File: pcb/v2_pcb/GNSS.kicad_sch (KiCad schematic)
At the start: 22 parts, among them J900 U.FL / Beitian BT-T076, U900 UM980

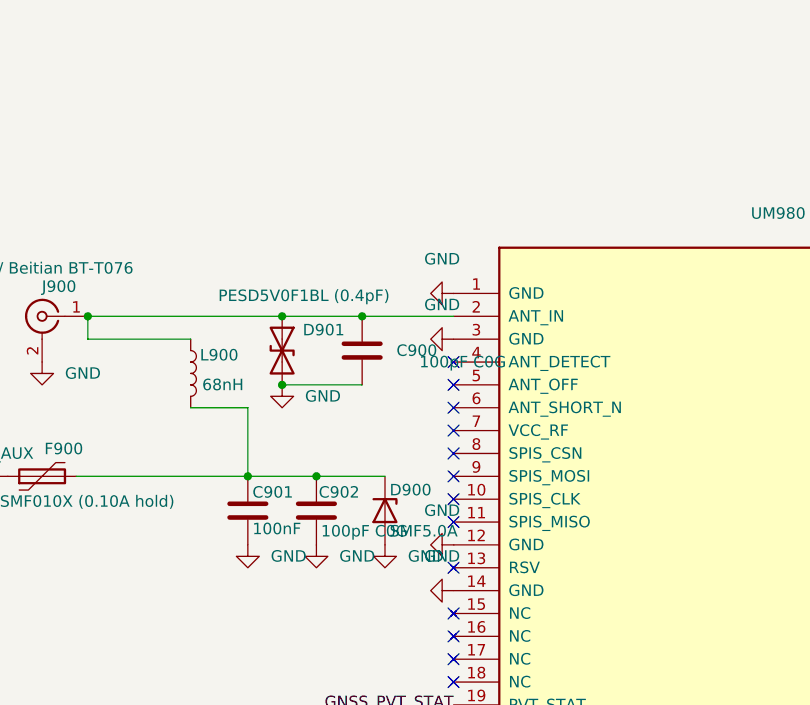
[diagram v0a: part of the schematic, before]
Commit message: fix minor
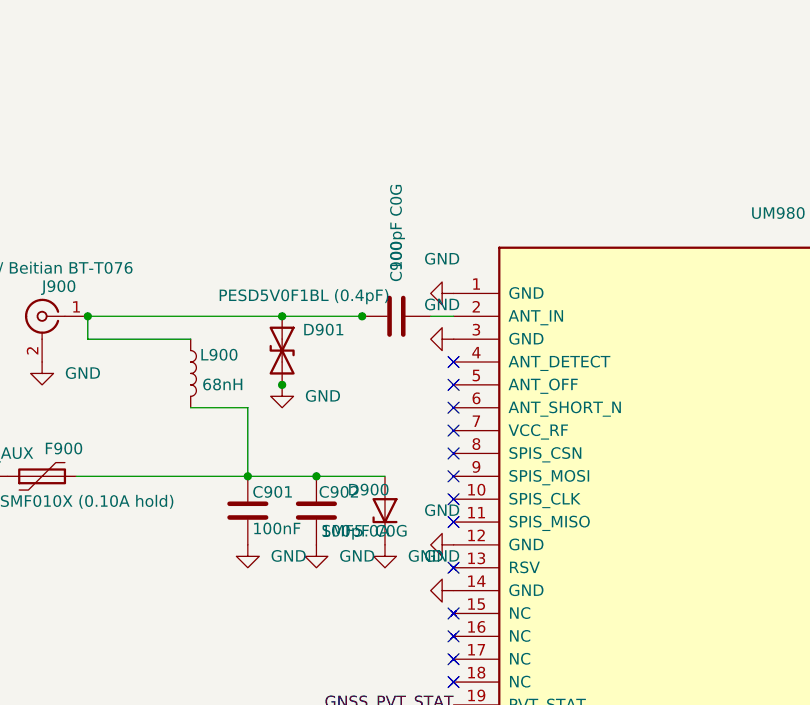
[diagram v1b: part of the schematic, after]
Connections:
- net GND: now also D900.1 (K); no longer C900.2, D900.2 (A)
- net at C901.1, C902.1, F900.2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: now also D900.2 (A); no longer D900.1 (K)
- net at C900.1, D901.1 (A1), J900.1 (In)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: no longer U900.2 (ANT_IN)
- new net: C900.2, U900.2 (ANT_IN)
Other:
- moved on the sheet: C900, D900
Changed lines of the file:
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@@
 	(wire
 		(pts
-			(xy 162.56 104.14) (xy 171.45 104.14)
-		)
-		(stroke
-			(width 0)
-			(type default)
-		)
-	)
-	(wire
-		(pts
 			(xy 323.85 146.05) (xy 349.25 146.05)
 		)
@@
 	(wire
 		(pts
-			(xy 171.45 96.52) (xy 181.61 96.52)
+			(xy 179.07 96.52) (xy 181.61 96.52)
 		)
 		(stroke
@@
 	(symbol
 		(lib_id "Device:D_Zener")
-		(at 173.99 118.11 270)
+		(at 173.99 118.11 90)
 		(unit 1)
 		(body_style 1)
@@
 	(symbol
 		(lib_id "Device:C")
-		(at 171.45 100.33 0)
+		(at 175.26 96.52 90)
 		(unit 1)
 		(body_style 1)
@@
 		(dnp no)
 		(property "Reference" "C900"
-			(at 175.26 100.33 0)
+			(at 175.26 92.71 0)
 			(show_name no)
 			(do_not_autoplace no)
@@
 		)
 		(property "Value" "100pF C0G"
-			(at 177.8 101.6 0)
+			(at 175.26 91.44 0)
 			(show_name no)
 			(do_not_autoplace no)
